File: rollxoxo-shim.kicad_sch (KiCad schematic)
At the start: 60 parts, among them J1 Conn_01x10, J2 USB_C_Receptacle_USB2.0_14P, J3 Conn_01x02, J4 Conn_01x04_Pin, J5 Conn_01x01, J6 Conn_01x10, SW1 SW_Push, SW2 SW_Push, U1 SN74LV1T125DBV, U2 ESP32-S3FN8, U3 SN74LV1T125DBV, U4 SN74LV1T125DBV, U6 SN74LV1T125DBV, Y1 48M

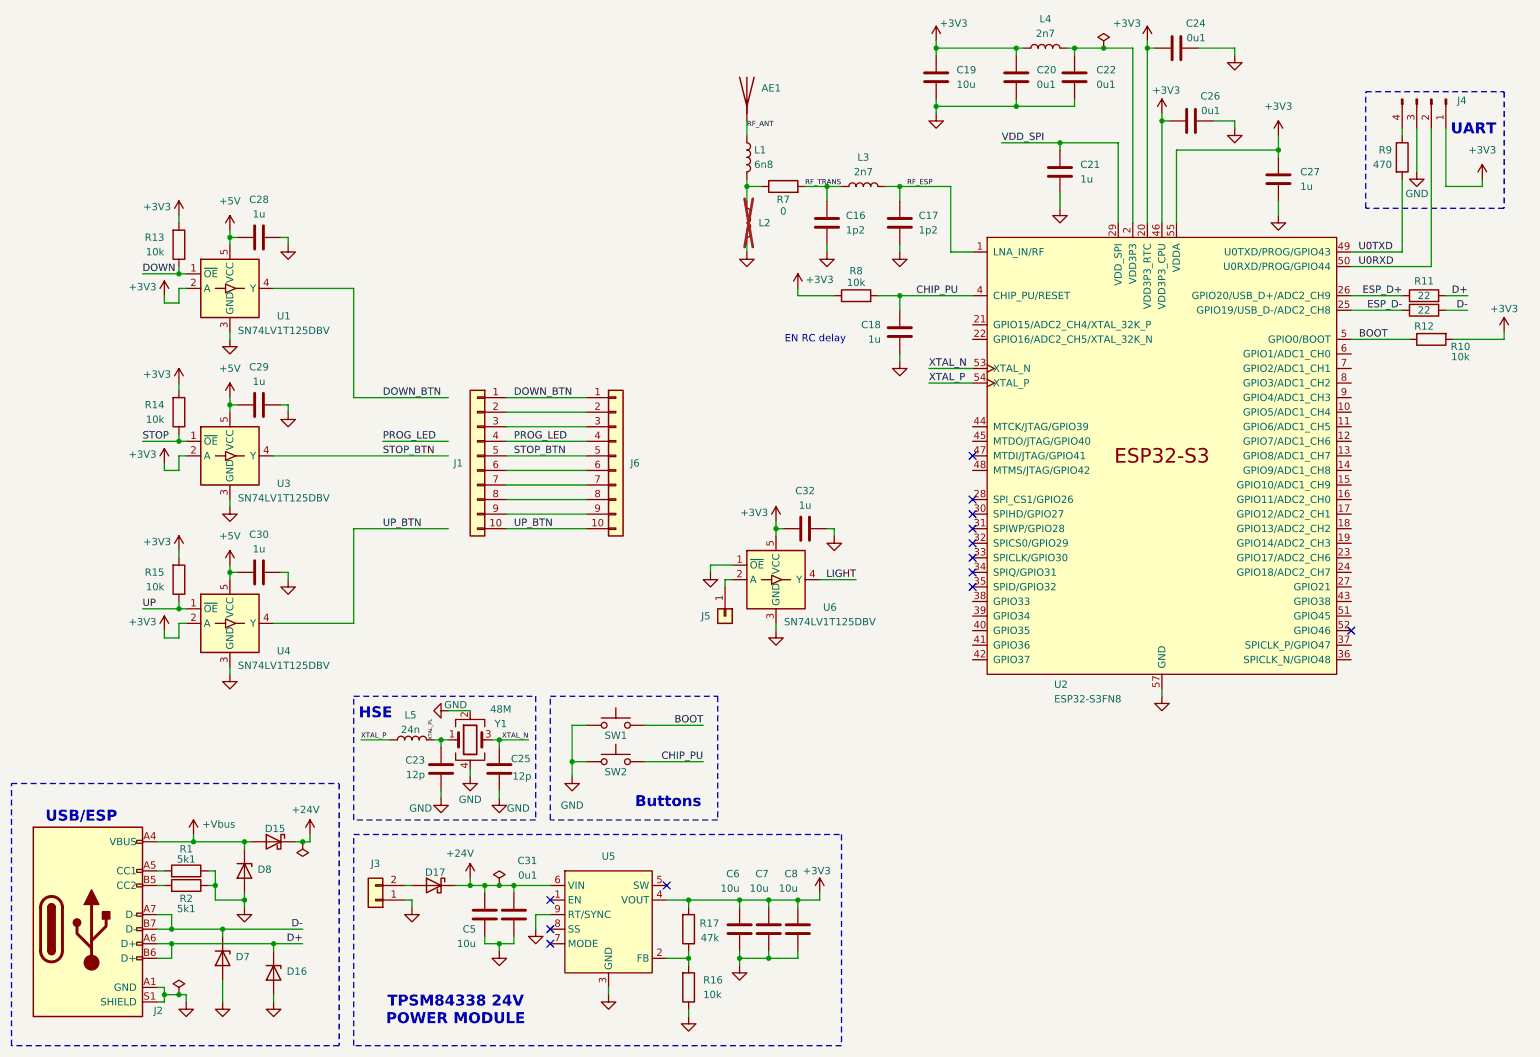
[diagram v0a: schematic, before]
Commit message: schem: reorganize
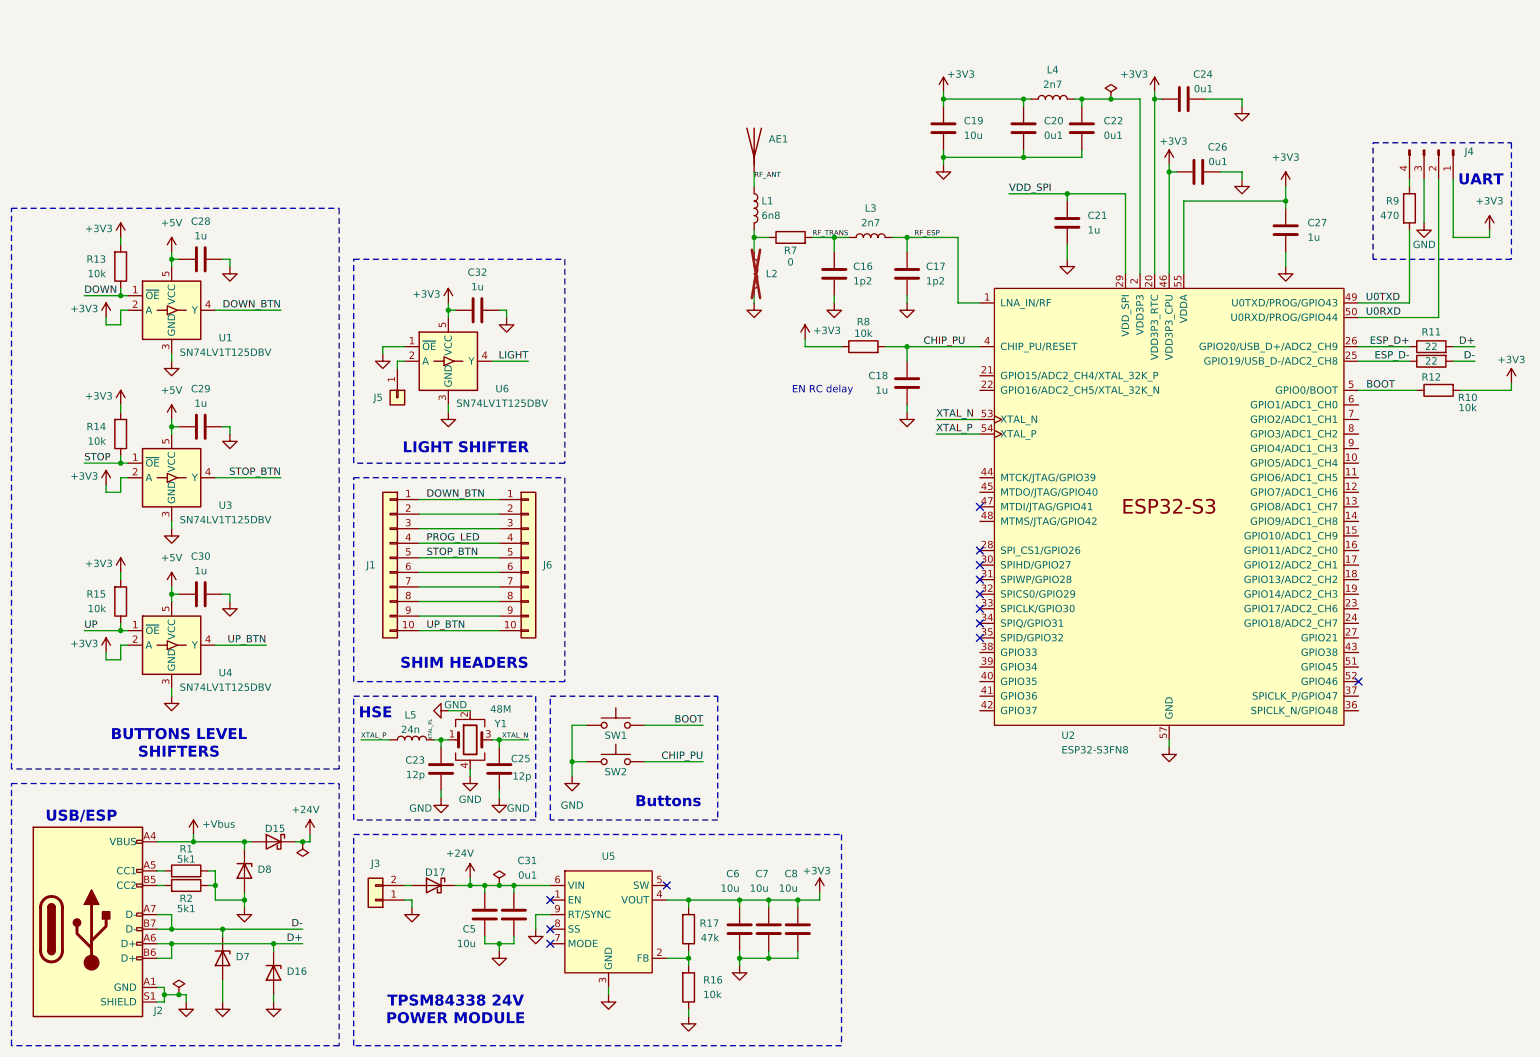
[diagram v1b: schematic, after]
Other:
- note added: "BUTTONS LEVEL SHIFTERS"
- note added: "LIGHT SHIFTER"
- note added: "SHIM HEADERS"
- moved on the sheet: AE1, C16, C17, C18, C19, C20, C21, C22, C24, C26, C27, C28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
